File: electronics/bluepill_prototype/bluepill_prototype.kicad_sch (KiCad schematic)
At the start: 16 parts, among them K1 Fujitsu_FTR-LYCA005x, M1 Motor_DC, SW1 SW_SPST, U1 Open_drain_hall_sensor, U2 YAAJ_BluePill_Part_Like, U3 MCP40D17

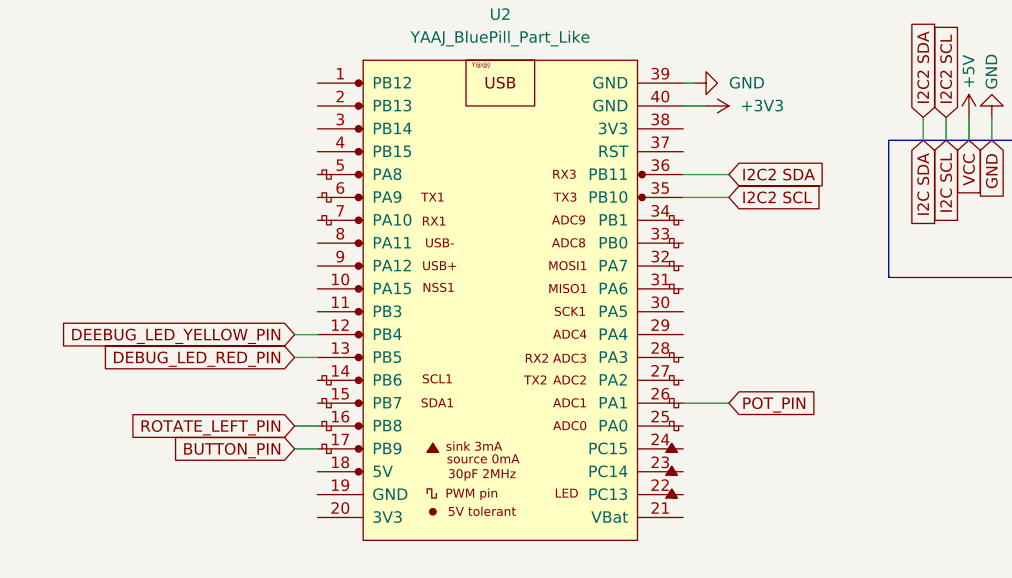
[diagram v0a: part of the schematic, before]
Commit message: fixed schematic
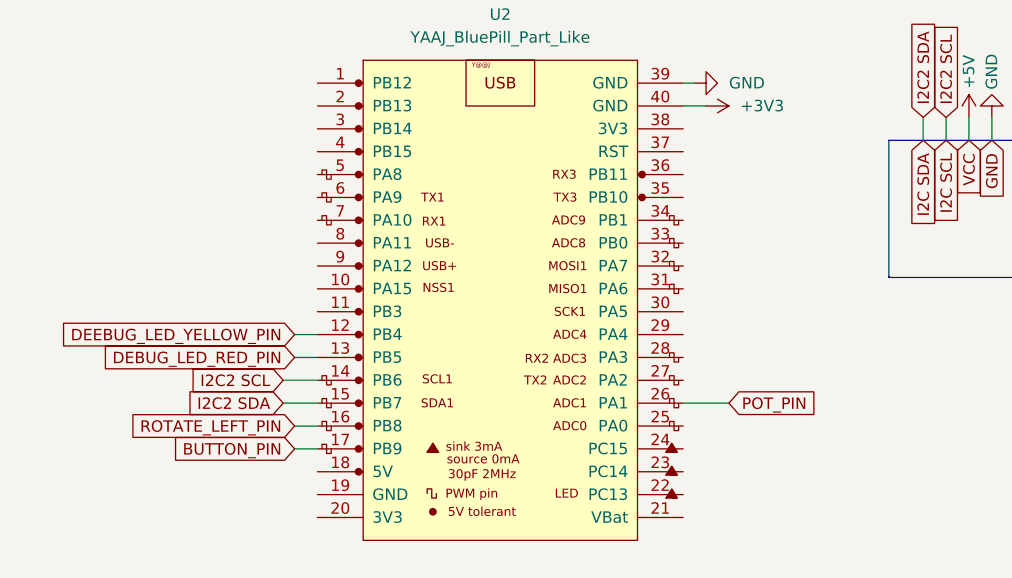
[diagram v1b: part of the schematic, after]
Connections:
- net I2C SCL: now also U2.14 (PB6); no longer U2.35 (PB10)
- net I2C SDA: now also U2.15 (PB7); no longer U2.36 (PB11)
